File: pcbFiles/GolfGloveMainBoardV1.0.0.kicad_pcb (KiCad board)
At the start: 4 copper layers, 55.3 x 40 mm, 137 parts, among them J1 USB_C_Receptacle, J14 Conn_01x02, J15 Conn_01x02, J16 Conn_01x02, J17 Conn_01x02, J2 Conn_01x06, J3 USB_C_Receptacle, J4 Conn_01x02_Male, J5 Conn_01x02_Male, J6 Conn_01x02_Male, J7 Conn_01x02, J8 Conn_01x02, J9 Conn_01x02, SW1 SW_SPDT, SW2 SW_Push, SW3 SW_Push_Dual, U1 MCP73831T-2ACI/OT, U3 LSM9DS1TR, U4 CYW20719B1KUMLG, U5 LSM9DS1TR, U7 TPS63001DRCT, Y1 Crystal, Y3 Crystal_GND24

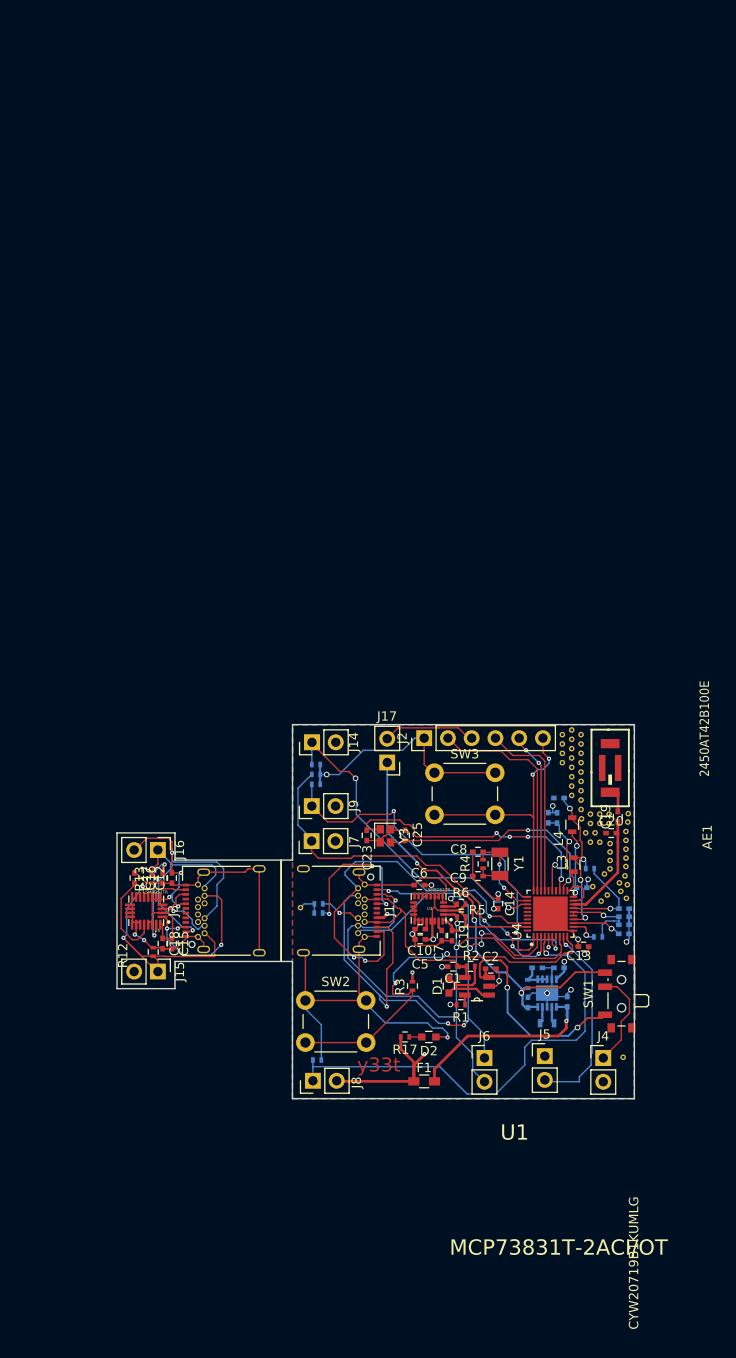
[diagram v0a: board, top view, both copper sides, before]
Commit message: Update To Rev3
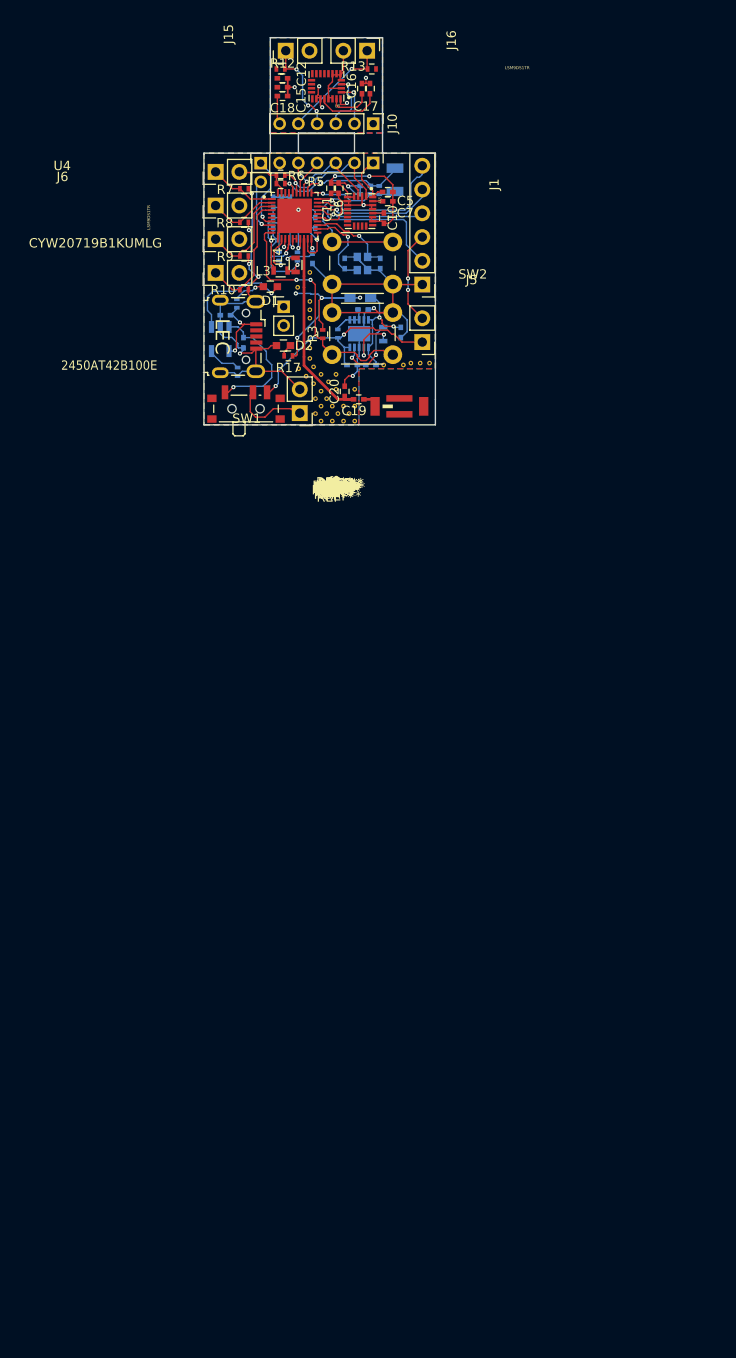
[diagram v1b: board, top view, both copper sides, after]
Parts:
- removed R14, R16: R, Resistors_SMD:R_0402
- removed the REF** at (148.3, 120.9)
- removed the REF** at (148.1, 129.9)
- removed the REF** at (146.0, 129.6)
- removed the REF** at (145.4, 130.2)
- removed the REF** at (146.7, 128.9)
- removed the REF** at (141.2, 113.4)
- removed the REF** at (141.2, 115.4)
- removed the REF** at (141.2, 112.4)
- removed the REF** at (145.7, 127.3)
- removed the REF** at (148.2, 128.5)
- removed the REF** at (144.7, 122.9)
- removed the REF** at (147.3, 128.3)
- removed the REF** at (146.3, 126.8)
- removed the REF** at (143.7, 122.9)
- removed the REF** at (145.2, 123.9)
- removed the REF** at (141.2, 114.4)
- removed the REF** at (144.2, 123.9)
- removed the REF** at (146.3, 125.9)
- removed the REF** at (148.0, 123.7)
- removed the REF** at (148.0, 122.8)
- removed the REF** at (145.2, 121.9)
- removed the REF** at (145.2, 120.9)
- removed the REF** at (146.9, 130.0)
- removed the REF** at (144.2, 120.9)
- removed the REF** at (147.5, 129.2)
- removed the REF** at (148.2, 121.8)
- removed the REF** at (146.2, 121.9)
- removed the REF** at (144.2, 121.9)
- removed the REF** at (143.2, 120.4)
- removed the REF** at (148.0, 126.5)
- removed the REF** at (144.5, 125.7)
- removed the REF** at (146.2, 120.9)
- removed the REF** at (142.2, 113.9)
- removed the REF** at (143.3, 121.4)
- removed the REF** at (142.2, 117.9)
- removed the REF** at (147.9, 127.5)
- removed the REF** at (148.0, 125.6)
- removed the REF** at (142.2, 118.9)
- removed the REF** at (143.2, 119.4)
- removed the REF** at (142.2, 115.9)
- removed the REF** at (146.3, 125.0)
- removed the REF** at (142.2, 116.9)
- removed the REF** at (142.2, 111.9)
- removed the REF** at (142.2, 112.9)
- removed the REF** at (146.3, 124.1)
- removed the REF** at (143.2, 112.4)
- removed the REF** at (143.2, 113.4)
- removed the REF** at (143.2, 114.4)
- removed the REF** at (143.2, 115.4)
- removed the REF** at (143.2, 116.4)
- removed the REF** at (143.2, 117.4)
- removed the REF** at (143.2, 118.4)
- removed the REF** at (142.2, 114.9)
- removed the REF** at (144.5, 128.7)
- removed the REF** at (109.7, 131.9)
- removed the REF** at (144.2, 147.9)
- removed the REF** at (127.2, 118.9)
- added J10: Conn_01x06_Male, Pin_Headers:Pin_Header_Straight_1x06_Pitch2.00mm, F.Cu at (121.0, 47.1)
- added REF**: StitchingVias, StitchingVias, F.Cu at (113.0, 69.0)
- added REF**: StitchingVias, StitchingVias, F.Cu at (113.0, 72.4)
- added REF**: StitchingVias, StitchingVias, F.Cu at (114.2, 63.0)
- added REF**: StitchingVias, StitchingVias, F.Cu at (113.0, 73.3)
- added REF**: StitchingVias, StitchingVias, F.Cu at (114.2, 72.2)
- added REF**: StitchingVias, StitchingVias, F.Cu at (115.4, 78.9)
- added REF**: StitchingVias, StitchingVias, F.Cu at (116.6, 78.9)
- added REF**: StitchingVias, StitchingVias, F.Cu at (125.0, 72.7)
- added REF**: StitchingVias, StitchingVias, F.Cu at (126.0, 72.7)
- added REF**: StitchingVias, StitchingVias, F.Cu at (127.0, 72.7)
- added REF**: StitchingVias, StitchingVias, F.Cu at (118.4, 78.1)
- added REF**: StitchingVias, StitchingVias, F.Cu at (119.0, 75.5)
- added REF**: StitchingVias, StitchingVias, F.Cu at (117.8, 77.3)
- added REF**: StitchingVias, StitchingVias, F.Cu at (117.8, 78.9)
- added REF**: StitchingVias, StitchingVias, F.Cu at (124.2, 72.9)
- added REF**: StitchingVias, StitchingVias, F.Cu at (119.0, 78.9)
- added REF**: StitchingVias, StitchingVias, F.Cu at (113.8, 74.1)
- added REF**: StitchingVias, StitchingVias, F.Cu at (116.2, 74.7)
- added REF**: StitchingVias, StitchingVias, F.Cu at (115.4, 75.7)
- added REF**: StitchingVias, StitchingVias, F.Cu at (116.0, 78.1)
- added REF**: StitchingVias, StitchingVias, F.Cu at (119.0, 77.3)
- added REF**: StitchingVias, StitchingVias, F.Cu at (114.6, 73.1)
- added REF**: StitchingVias, StitchingVias, F.Cu at (117.0, 73.9)
- added REF**: StitchingVias, StitchingVias, F.Cu at (117.0, 75.5)
- added REF**: StitchingVias, StitchingVias, F.Cu at (114.8, 76.5)
- added REF**: StitchingVias, StitchingVias, F.Cu at (114.8, 78.1)
- added REF**: StitchingVias, StitchingVias, F.Cu at (117.2, 78.1)
- added REF**: StitchingVias, StitchingVias, F.Cu at (114.6, 74.9)
- added REF**: StitchingVias, StitchingVias, F.Cu at (115.4, 73.9)
- added REF**: StitchingVias, StitchingVias, F.Cu at (116.0, 76.5)
- added REF**: StitchingVias, StitchingVias, F.Cu at (115.4, 77.3)
- added REF**: StitchingVias, StitchingVias, F.Cu at (116.6, 77.3)
- added REF**: StitchingVias, StitchingVias, F.Cu at (114.2, 66.1)
- added REF**: StitchingVias, StitchingVias, F.Cu at (114.2, 67.9)
- added REF**: StitchingVias, StitchingVias, F.Cu at (114.2, 71.1)
- added REF**: StitchingVias, StitchingVias, F.Cu at (112.9, 64.6)
- added REF**: StitchingVias, StitchingVias, F.Cu at (114.2, 67.0)
- added REF**: StitchingVias, StitchingVias, F.Cu at (122.1, 72.9)
- AE1: footprint ANTENNA---------------------:XCVR_2450AT42B100E -> 2450AT42B100E:XCVR_2450AT42B100E
- C1, C13, C14, C2, C23, C25, C8, C9, F1, R1, R2, R4, U1, Y1, Y3: moved to B.Cu
- J1: value USB_C_Receptacle -> Conn_01x06_Male; footprint Connectors_USB:USB_C_Receptacle_Amphenol_12401548E4-2A -> Pin_Headers:Pin_Header_Straight_1x06_Pitch2.00mm
- J3: value USB_C_Receptacle -> USB_OTG; footprint Connectors_USB:USB_C_Receptacle_Amphenol_12401548E4-2A -> Connectors_USB:USB_Micro-B_Wuerth-629105150521
- J5, J6: footprint Pin_Headers:Pin_Header_Straight_1x02_Pitch2.54mm -> Pin_Headers:Pin_Header_Straight_1x02_Pitch2.00mm
- R10, R7, R8, R9: moved to F.Cu
- moved J15 99.4 mm to (111.7, 39.3), turned to 90 degrees
- moved J6 98.6 mm to (109.0, 51.3)
- moved R12 95.4 mm to (111.1, 41.2), turned to 0 degrees
- moved J8 94.2 mm to (104.2, 55.9)
- moved C15 93.3 mm to (111.3, 42.2), turned to 180 degrees
- moved C18 91.5 mm to (111.3, 44.1), turned to 180 degrees
- moved U5 90.2 mm to (116.0, 43.1)
- moved R8 89.9 mm to (107.2, 57.6)
- moved R13 89.7 mm to (120.8, 41.2), turned to 180 degrees
- moved J16 88.3 mm to (120.3, 39.3)
- moved C17 88.1 mm to (120.7, 43.4)
- moved C16 87.1 mm to (119.8, 43.4), turned to 270 degrees
- moved C22 86.7 mm to (110.3, 55.5), turned to 270 degrees
- moved C13 85.9 mm to (111.2, 55.5), turned to 90 degrees
- moved C12 85.4 mm to (111.3, 43.2), turned to 0 degrees
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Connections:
- J5 pad 1: Net-(J5-Pad1) -> SCLK
- J5 pad 2: Net-(J5-Pad2) -> SDA
- J6 pad 1: SDA -> Net-(J6-Pad1)
- J6 pad 2: SCLK -> Net-(J6-Pad2)
- U4 pad 1: Sensor3 -> Sensor1
- U4 pad 2: SDA -> Sensor2
- U4 pad 3: Sensor1 -> Sensor3
- U4 pad 33: Sensor4 -> PSensor2
- U4 pad 34: Net-(U4-Pad34) -> PSensor1
- U4 pad 35: Net-(U4-Pad35) -> SDA
- U4 pad 36: Net-(U4-Pad36) -> SCLK
- U4 pad 38: PSensor1 -> Net-(U4-Pad38)
- U4 pad 4: Sensor2 -> Sensor4
- U4 pad 5: Net-(J5-Pad1) -> Net-(U4-Pad5)
- U4 pad 6: PSensor2 -> Net-(U4-Pad6)
- U4 pad 7: Net-(U4-Pad7) -> Net-(J6-Pad1)
- U4 pad 8: SCLK -> Net-(J6-Pad2)
- U4 pad 9: Net-(J5-Pad2) -> Net-(U4-Pad9)
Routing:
- net 3.3v: track 352.4 -> 105.9 mm, vias 11 -> 6
- net PSensor1: track 74.5 -> 14.1 mm, vias 5 -> 3
- net PSensor2: track 57.8 -> 15.6 mm
- net Sensor2: track 49.7 -> 7.61 mm, vias 1 -> 0
- net Sensor1: track 42.1 -> 7.20 mm, vias 4 -> 0
- net SDA: track 69.9 -> 35.2 mm, vias 7 -> 1
- net SCLK: track 63.1 -> 30.2 mm, vias 3 -> 1
- net Sensor3: track 40.9 -> 11.0 mm, vias 2 -> 0
- net USBVCC: track 40.9 -> 14.9 mm, vias 4 -> 2
- net USBGND: track 39.8 -> 13.9 mm, vias 2 -> 3
- net BatteryOutBuck: track 47.4 -> 24.8 mm, vias 3 -> 2
- net Sensor4: track 35.2 -> 13.8 mm, vias 2 -> 0
- net Net-(J5-Pad2): track 21.2 -> 0.00 mm, vias 1 -> 0
- net Net-(C23-Pad1): track 29.7 -> 9.08 mm, vias 4 -> 1
- net Net-(J5-Pad1): track 20.0 -> 0.00 mm, vias 1 -> 0
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- added copper zone on B.Cu, net USBGND
- added copper zone on F.Cu, net USBGND
- added copper zone on In2.Cu, net USBGND
- added copper zone on In1.Cu, net USBVCC
- removed copper zone on In1.Cu, net USBGND
- removed copper zone on In2.Cu, net USBVCC
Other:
- board size 55.3 x 40 mm -> 24.8 x 41.4 mm
- board text removed: "Golf Glove"
- board text removed: "REV1.0"
- board text removed: "REV2.0"
- board text removed: "y33t"
